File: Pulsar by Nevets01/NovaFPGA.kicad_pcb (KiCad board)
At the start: 2 copper layers, 381 x 140.3 mm, 82 parts, among them J1 Conn_02x32_Odd_Even, J10 Conn_02x38_Odd_Even, J11 MAX3223, J12 Conn_01x03, J13 Conn_01x03, J14 Conn_01x06_Male, J15 Conn_01x06_Male, J2 Conn_02x32_Odd_Even, J3 SD_Card, J4 Conn_02x50_Even_Odd, J5 Conn_02x50_Even_Odd, J6 Conn_01x04, J7 Conn_01x03, J8 Conn_01x02, J9 Conn_01x01, U1 74LS03, U10 74LS03, U11 74LS00, U12 74LS02, U13 74LS03, U14 74LS03, U15 74LS03, U16 74LS03, U17 74LS03, U18 74LVCH16240, U19 LM1117-3.3, U2 74LS03, U3 74LS03, U4 74LS03, U5 74LS03, U6 74LS03, U7 74LVCH16240, U8 74LVCH16240, U9 74LVCH16240

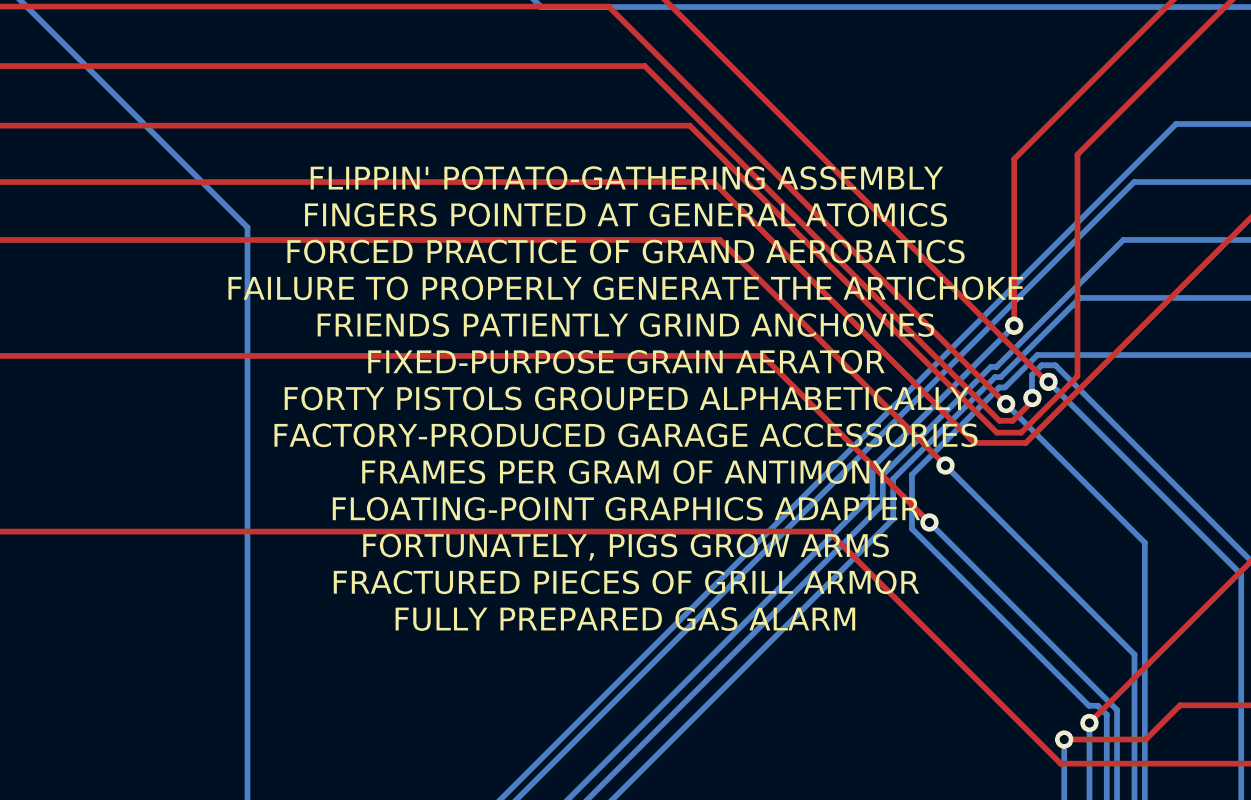
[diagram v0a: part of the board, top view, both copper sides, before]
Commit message: Mod
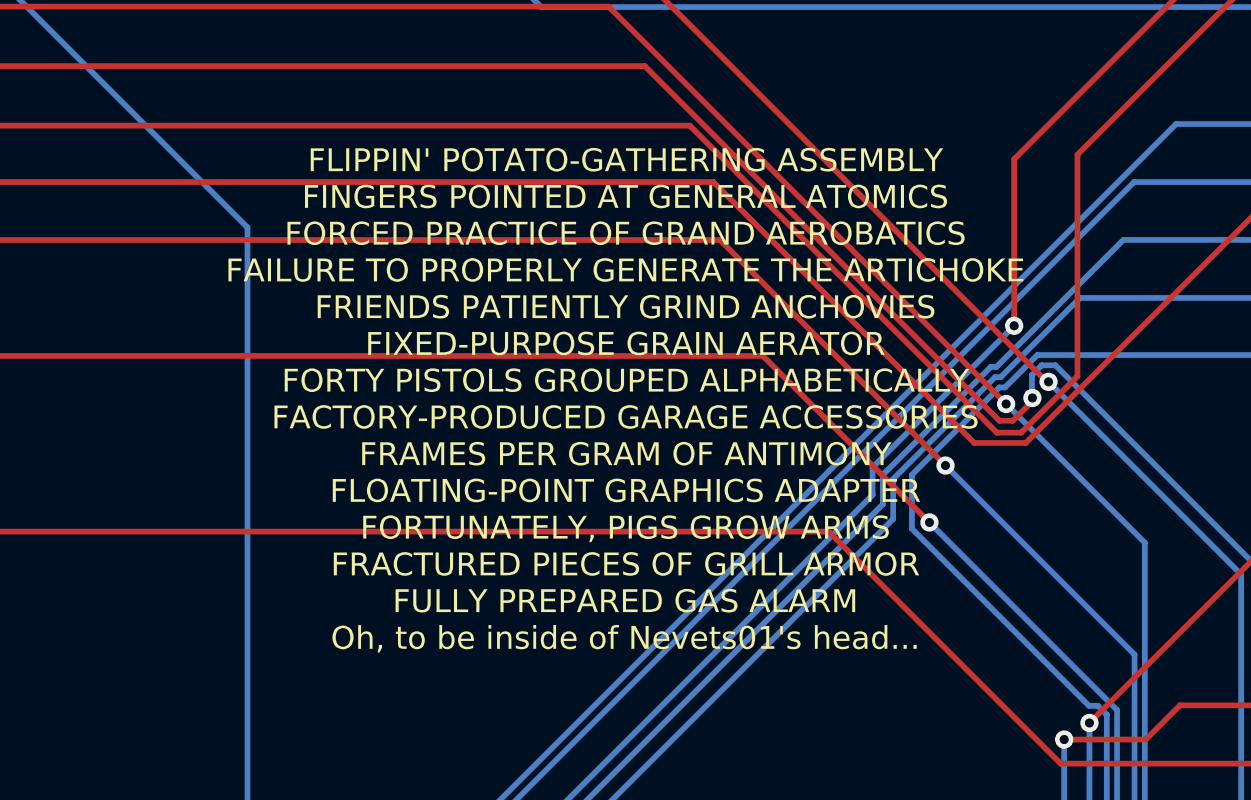
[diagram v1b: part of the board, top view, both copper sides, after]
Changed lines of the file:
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@@
     (effects (font (size 1 1) (thickness 0.15)))
   )
-  (gr_text "FLIPPIN' POTATO-GATHERING ASSEMBLY\nFINGERS POINTED AT GENERAL ATOMICS\nFORCED PRACTICE OF GRAND AEROBATICS\nFAILURE TO PROPERLY GENERATE THE ARTICHOKE\nFRIENDS PATIENTLY GRIND ANCHOVIES\nFIXED-PURPOSE GRAIN AERATOR\nFORTY PISTOLS GROUPED ALPHABETICALLY\nFACTORY-PRODUCED GARAGE ACCESSORIES\nFRAMES PER GRAM OF ANTIMONY\nFLOATING-POINT GRAPHICS ADAPTER\nFORTUNATELY, PIGS GROW ARMS\nFRACTURED PIECES OF GRILL ARMOR\nFULLY PREPARED GAS ALARM" (at 213.614 76.073) (layer "F.SilkS")
+  (gr_text "FLIPPIN' POTATO-GATHERING ASSEMBLY\nFINGERS POINTED AT GENERAL ATOMICS\nFORCED PRACTICE OF GRAND AEROBATICS\nFAILURE TO PROPERLY GENERATE THE ARTICHOKE\nFRIENDS PATIENTLY GRIND ANCHOVIES\nFIXED-PURPOSE GRAIN AERATOR\nFORTY PISTOLS GROUPED ALPHABETICALLY\nFACTORY-PRODUCED GARAGE ACCESSORIES\nFRAMES PER GRAM OF ANTIMONY\nFLOATING-POINT GRAPHICS ADAPTER\nFORTUNATELY, PIGS GROW ARMS\nFRACTURED PIECES OF GRILL ARMOR\nFULLY PREPARED GAS ALARM\nOh, to be inside of Nevets01's head..." (at 213.614 76.073) (layer "F.SilkS")
     (effects (font (size 1 1) (thickness 0.15)))
   )
